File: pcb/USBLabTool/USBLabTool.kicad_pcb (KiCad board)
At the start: 4 copper layers, 79.4 x 56.2 mm, 250 parts, among them J1 Conn_01x06_Pin, J17 2x01, J19 T_N5V, J2 Conn_02x12_Odd_Even, J20 USB_C_Receptacle, K1 G5V-2, K2 G5V-2, Q1 STL11N3LLH6, SW1 TS02-66-73-BK-100-SCR-D, U1 AQY284SX, U10 MC33274ADR2G, U11 DG403, U12 STM32H563VITx, U13 R1283K002A, U14 ST1L05APU33R, U15 ST1L05APU33R, U16 LTC1983ES6-5TRMPBF, U17 TCPP01-M12, U18 74HC245, U19 USBLC6-2SC6, U2 AQY284SX, U20 74HC245, U3 CD74HC4316, U4 LMP7718, U5 CD74HC4316, U6 LMP7718, U7 OPA863, U8 OPA863, U9 MC33274ADR2G, Y1 32.768kHz, Y2 NX2016SA-25M-EXS00A-CS08742

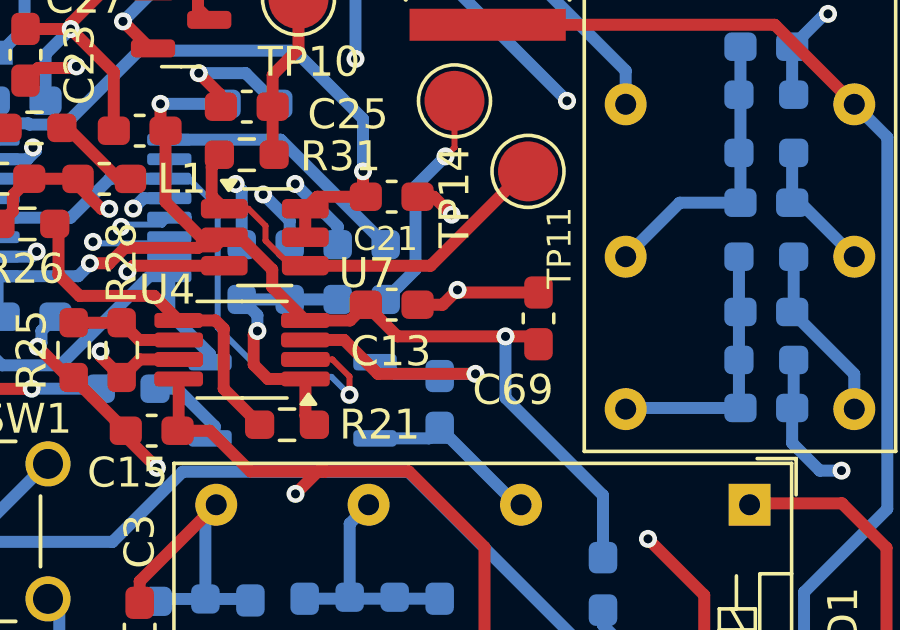
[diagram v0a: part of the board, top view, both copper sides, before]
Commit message: update pcb v2
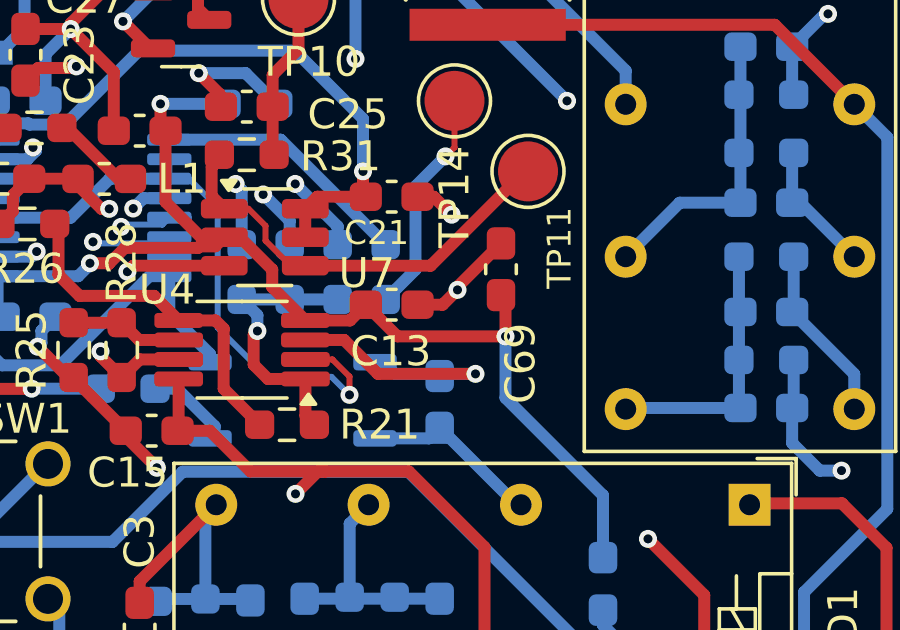
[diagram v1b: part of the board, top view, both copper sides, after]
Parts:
- moved C69 2.06 mm to (175.3, 89.3)
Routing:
- net GNDA: track 314.8 -> 314.2 mm
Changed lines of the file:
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@@
 	(footprint "Capacitor_SMD:C_0603_1608Metric_Pad1.08x0.95mm_HandSolder"
 		(layer "F.Cu")
-		(at 176.6 90.9 90)
+		(at 175.35 89.2625 90)
 		(descr "Capacitor SMD 0603 (1608 Metric), square (rectangular) end terminal, IPC-7351 nominal with elongated pad for handsoldering. (Body size source: IPC-SM-782 page 76, https://www.pcb-3d.com/wordpress/wp-content/uploads/ipc-sm-782a_amendment_1_and_2.pdf), generated with kicad-footprint-generator")
 		(tags "capacitor handsolder")
 		(property "Reference" "C69"
-			(at -2.3875 -0.85 180)
+			(at -3.1375 0.65 270)
 			(layer "F.SilkS")
 			(effects
@@
 		(tags "capacitor handsolder")
 		(property "Reference" "C21"
-			(at 0.206 -1.406 180)
+			(at 0.506 -1.206 180)
 			(layer "F.SilkS")
 			(effects
@@
 	)
 	(segment
-		(start 176.6 90.0375)
-		(end 173.9875 90.0375)
-		(width 0.4)
-		(layer "F.Cu")
-		(net 2)
-	)
-	(segment
 		(start 131.089 81.075)
 		(end 135.6125 81.075)
@@
 	)
 	(segment
+		(start 173.9 89.85)
+		(end 175.35 88.4)
+		(width 0.4)
+		(layer "F.Cu")
+		(net 2)
+	)
+	(segment
 		(start 123.015 105.515)
 		(end 124.225 105.515)
@@
 	)
 	(segment
+		(start 173.9 89.95)
+		(end 173.9 89.85)
+		(width 0.4)
+		(layer "F.Cu")
+		(net 2)
+	)
+	(segment
 		(start 174.906 76.9739)
 		(end 175.7761 76.9739)
@@
 	)
 	(segment
-		(start 173.9875 90.0375)
-		(end 173.9 89.95)
-		(width 0.4)
-		(layer "F.Cu")
-		(net 2)
-	)
-	(segment
 		(start 130 82.164)
 		(end 130 83.809999)
@@
 	)
 	(segment
-		(start 175.5 91.5)
-		(end 176.3375 91.5)
+		(start 150.6375 78.648)
+		(end 149.351 77.3615)
 		(width 0.4)
 		(layer "F.Cu")
@@
 	)
 	(segment
-		(start 150.6375 78.648)
-		(end 149.351 77.3615)
+		(start 168.831 90.969)
+		(end 170.3185 90.969)
 		(width 0.4)
 		(layer "F.Cu")
@@
 	)
 	(segment
-		(start 168.831 90.969)
-		(end 170.3185 90.969)
+		(start 175.5 90.275)
+		(end 175.35 90.125)
 		(width 0.4)
 		(layer "F.Cu")
@@
 	)
 	(segment
-		(start 176.3375 91.5)
-		(end 176.6 91.7625)
-		(width 0.4)
-		(layer "F.Cu")
-		(net 18)
-	)
-	(segment
 		(start 164 83.75)
 		(end 164 84.4755)
@@
 		(width 0.4)
 		(layer "F.Cu")
+		(net 18)
+	)
+	(segment
+		(start 175.5 91.5)
+		(end 175.5 90.275)
+		(width 0.4)
+		(layer "F.Cu")
